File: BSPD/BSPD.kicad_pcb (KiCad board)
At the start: 2 copper layers, 160 x 124.7 mm, 41 parts, among them J1 DT13-48PABCD-R015, K1 Latching Relay, Q1 STS6NF20V, Q2 STS6NF20V, Q3 STS6NF20V, U1 LM7805CT, U10 DK1A1B-12V, U11 NSL-32, U12 LM555N, U13 LM7805CT, U2 OP AMP, U3 OP AMP, U4 Inverter (Not Gate), U5 2x4 OR GATE, U6 LM555N, U7 NSL-32, U8 NAND, U9 AND GATE

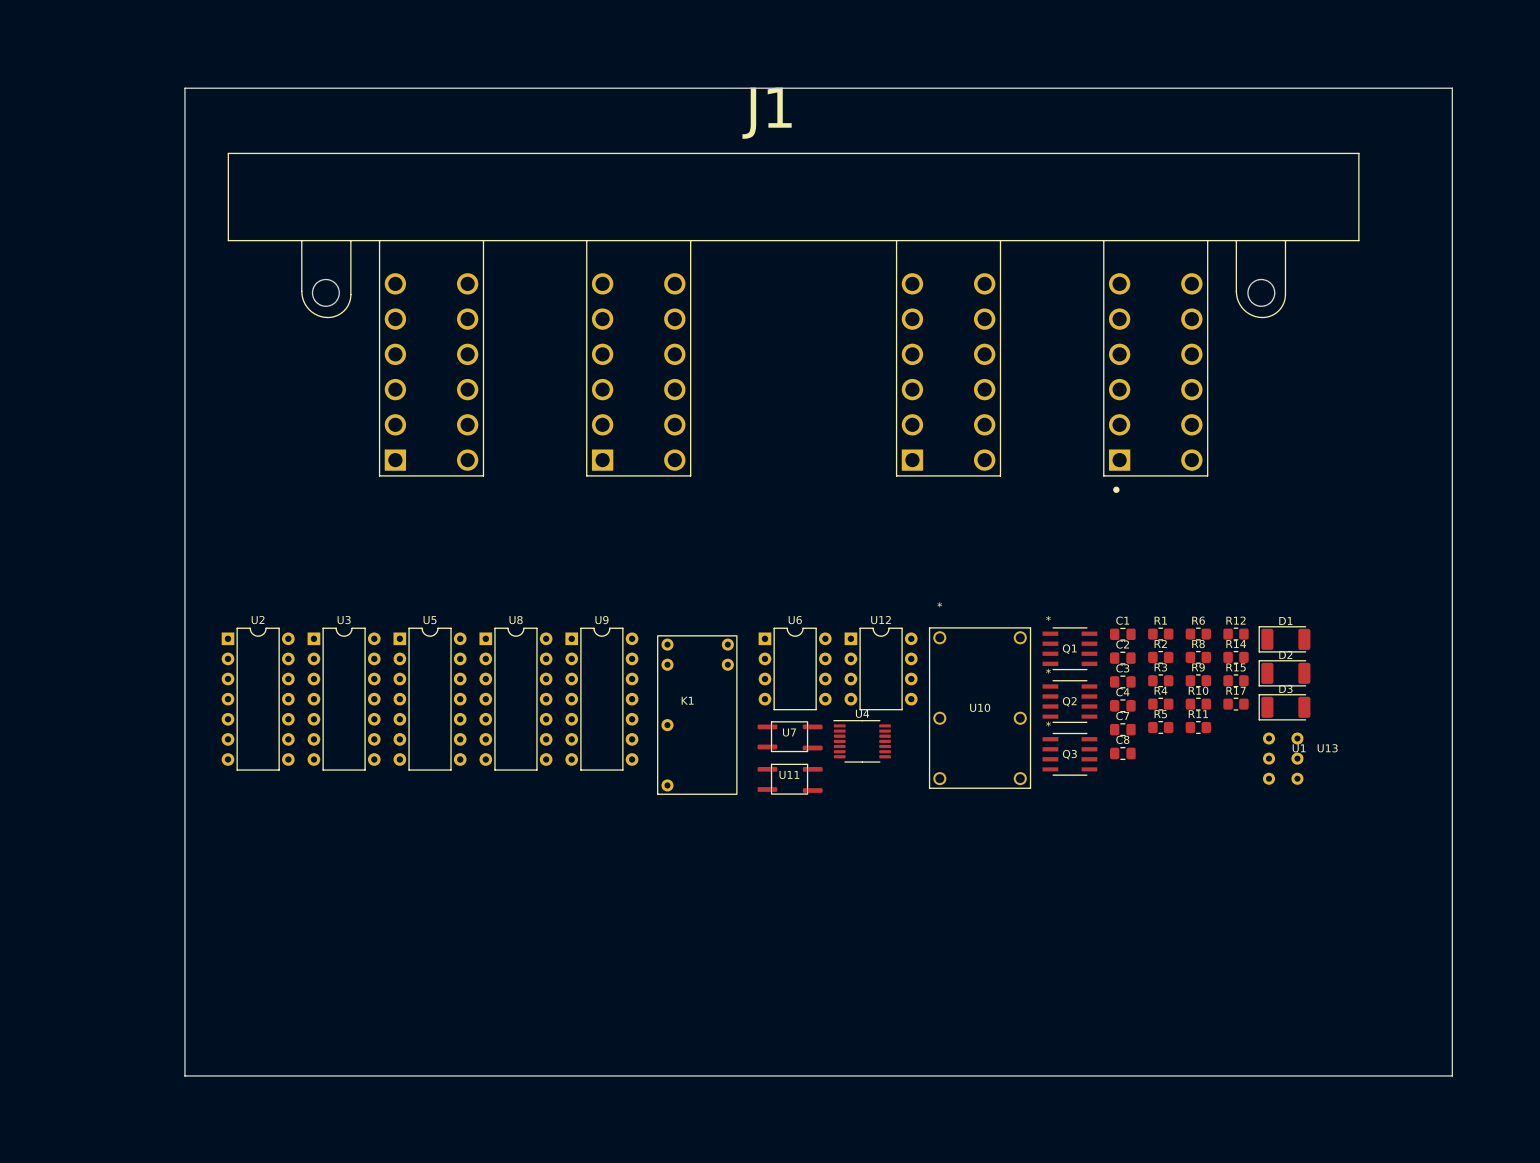
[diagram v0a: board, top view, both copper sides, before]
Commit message: 1/2 BSPD Circuitry
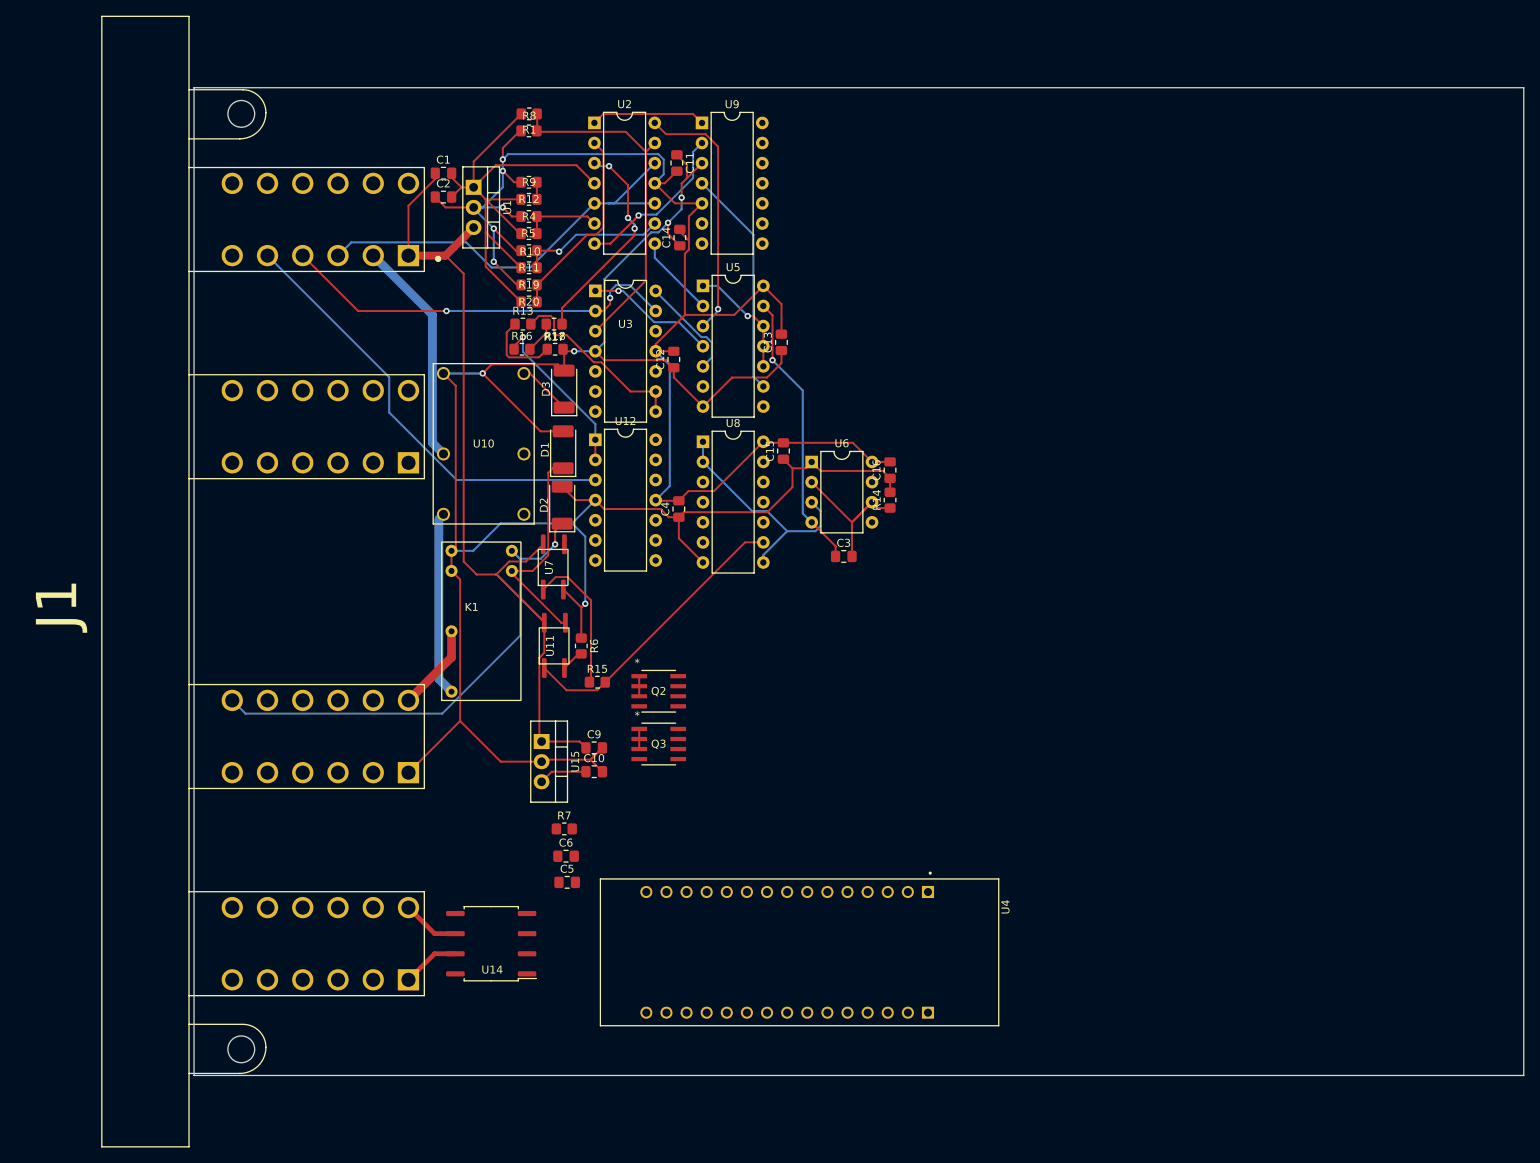
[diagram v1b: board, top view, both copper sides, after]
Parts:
- removed C7: 330nf, Capacitor_SMD:C_0805_2012Metric_Pad1.18x1.45mm_HandSolder
- removed C8: 100nf, Capacitor_SMD:C_0805_2012Metric_Pad1.18x1.45mm_HandSolder
- removed Q1: STS6NF20V, 1FS_2_Global_Footprint_Library:SO-8_STM
- removed R2: 18k, Resistor_SMD:R_0805_2012Metric_Pad1.20x1.40mm_HandSolder
- removed R3: 2.7k, Resistor_SMD:R_0805_2012Metric_Pad1.20x1.40mm_HandSolder
- removed U13: LM7805CT, 1FS_2_Global_Footprint_Library:Basic 3 Hole
- added C10: 0.33µF, Capacitor_SMD:C_0805_2012Metric_Pad1.18x1.45mm_HandSolder, F.Cu at (77.6, 109.2)
- added C11: 100nf, Capacitor_SMD:C_0805_2012Metric_Pad1.18x1.45mm_HandSolder, F.Cu at (88.0, 32.4)
- added C12: 100nf, Capacitor_SMD:C_0805_2012Metric_Pad1.18x1.45mm_HandSolder, F.Cu at (87.6, 57.2)
- added C13: 100nf, Capacitor_SMD:C_0805_2012Metric_Pad1.18x1.45mm_HandSolder, F.Cu at (101.2, 55.0)
- added C14: 100nf, Capacitor_SMD:C_0805_2012Metric_Pad1.18x1.45mm_HandSolder, F.Cu at (88.4, 41.8)
- added C15: 100nf, Capacitor_SMD:C_0805_2012Metric_Pad1.18x1.45mm_HandSolder, F.Cu at (101.5, 68.7)
- added C16: 100nf, Capacitor_SMD:C_0805_2012Metric_Pad1.18x1.45mm_HandSolder, F.Cu at (114.9, 71.1)
- added C5: 100nF, Capacitor_SMD:C_0805_2012Metric_Pad1.18x1.45mm_HandSolder, F.Cu at (74.2, 123.2)
- added C6: 100nF, Capacitor_SMD:C_0805_2012Metric_Pad1.18x1.45mm_HandSolder, F.Cu at (74.0, 119.9)
- added C9: 0.33µF, Capacitor_SMD:C_0805_2012Metric_Pad1.18x1.45mm_HandSolder, F.Cu at (77.6, 106.2)
- added R13: 39k, Resistor_SMD:R_0805_2012Metric_Pad1.20x1.40mm_HandSolder, F.Cu at (68.6, 52.7)
- added R16: 39k, Resistor_SMD:R_0805_2012Metric_Pad1.20x1.40mm_HandSolder, F.Cu at (68.5, 55.9)
- added R18: 1M, Resistor_SMD:R_0805_2012Metric_Pad1.20x1.40mm_HandSolder, F.Cu at (72.6, 55.9)
- added R19: 22k 1%, Resistor_SMD:R_0805_2012Metric_Pad1.20x1.40mm_HandSolder, F.Cu at (69.4, 47.8)
- added R20: 18k 1%, Resistor_SMD:R_0805_2012Metric_Pad1.20x1.40mm_HandSolder, F.Cu at (69.4, 49.9)
- added R7: 120, Resistor_SMD:R_0805_2012Metric_Pad1.20x1.40mm_HandSolder, F.Cu at (73.8, 116.4)
- added U14: ISO1050DUB, Package_SO:SOP-8_6.62x9.15mm_P2.54mm, F.Cu at (64.6, 130.9)
- added U15: LM7809_TO220, Package_TO_SOT_THT:TO-220-3_Vertical, F.Cu at (70.9, 105.4)
- C4: value 1uf -> 100nf
- R17: value 2.4M -> 1M
- U1: footprint 1FS_2_Global_Footprint_Library:Basic 3 Hole -> Package_TO_SOT_THT:TO-220-3_Vertical
- U12: value LM555N -> OP AMP; footprint Package_DIP:DIP-8_W7.62mm -> Package_DIP:DIP-14_W7.62mm
- U4: value Inverter (Not Gate) -> NUCLEO-L432KC; footprint Package_SO:TSSOP-14_4.4x5mm_P0.65mm -> 1FS_2_Global_Footprint_Library:MODULE_NUCLEO-L432KC
- moved U1 123.6 mm to (62.4, 35.4), turned to -90 degrees
- moved R8 108.8 mm to (69.4, 26.2), turned to 180 degrees
- moved R9 105.4 mm to (69.3, 34.8), turned to 180 degrees
- moved R12 104.8 mm to (69.3, 37.0)
- moved C1 103.7 mm to (58.5, 33.7)
- moved C2 103.7 mm to (58.5, 36.7)
- moved R11 102.5 mm to (69.4, 45.6), turned to 180 degrees
- moved R10 102.1 mm to (69.3, 43.4)
- moved R1 102.0 mm to (69.3, 28.3)
- moved R5 101.3 mm to (69.3, 41.3), turned to 180 degrees
- moved R4 100.8 mm to (69.3, 39.1)
- moved D3 99.6 mm to (73.8, 60.9), turned to 90 degrees
- moved R17 98.6 mm to (72.5, 52.7), turned to 180 degrees
- moved D1 94.3 mm to (73.7, 68.6), turned to 90 degrees
- moved D2 93.8 mm to (73.5, 75.6), turned to 90 degrees
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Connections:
- net /4.1V renamed /Brake Threshhold (4.1V)
- net Net-(U2-Pad14) renamed /BrkSenShort
- net Net-(U2-Pad8) renamed /BrkSenOpen
- net Net-(U3-Pad1) renamed /CurSenShort
- net Net-(U3-Pad14) renamed /CurSenOpen
- C3 pad 1: Net-(U6-R) -> /BSPD Fault
- C4 pad 1: +5V -> GND
- C4 pad 2: Net-(U12-THR) -> +5V
- D1 pad 2: Net-(D1-A) -> GND
- J1 pad A10: /BMS_FAULT 3.3V -> unconnected-(J1-PadA10)
- J1 pad A11: /BMS Light Low Side -> unconnected-(J1-PadA11)
- J1 pad A12: /IMD Light Low Side -> unconnected-(J1-PadA12)
- J1 pad A2: unconnected-(J1-PadA2) -> /Shutdown In
- J1 pad A6: /SH_RESET -> unconnected-(J1-PadA6)
- J1 pad A8: /Shutdown In -> unconnected-(J1-PadA8)
- J1 pad A9: /IMD_FAULT -> unconnected-(J1-PadA9)
- J1 pad B1: unconnected-(J1-PadB1) -> /CAN_Tel_H
- J1 pad B12: unconnected-(J1-PadB12) -> /CAN_Tel_L
- J1 pad D10: unconnected-(J1-PadD10) -> /BMS Light Low Side
- J1 pad D11: unconnected-(J1-PadD11) -> /IMD Light Low Side
- J1 pad D12: unconnected-(J1-PadD12) -> /Shutdown Out
- J1 pad D3: /Shutdown Out -> unconnected-(J1-PadD3)
- J1 pad D7: unconnected-(J1-PadD7) -> /SH_RESET
- J1 pad D8: unconnected-(J1-PadD8) -> /IMD_FAULT 5V
- J1 pad D9: unconnected-(J1-PadD9) -> /BMS_FAULT 5V
- K1 pad 2: Net-(D1-A) -> GND
- R15 pad 2: /BSPD Fault -> /BSPD Fault Post Timer
- R17 pad 1: Net-(U12-THR) -> /Current Sensor Differential
- R17 pad 2: GND -> /Current Vref Op
- U11 pad 1: Net-(U11-A) -> /BSPD Fault Post Timer
- U12 pad 1: GND -> /Current Vref Buffered
- U12 pad 2: Net-(U12-THR) -> /Current Vref Buffered
- U12 pad 3: /IMD Latch Delay -> /Current Vref
- U12 pad 4: +5V -> GND
- U12 pad 6: Net-(U12-THR) -> unconnected-(U12-Pad6)
- U12 pad 8: +5V -> unconnected-(U12-Pad8)
- U2 pad 2: /Current Vref -> /2.25V
- U2 pad 3: /Current Output -> /Current Sensor Differential
- U2 pad 5: /Current Output -> /Brake Output
- U3 pad 10: /BMS_FAULT 3.3V -> /Current Output
- U3 pad 5: unconnected-(U3-Pad5) -> /Current Vref Op
- U3 pad 6: unconnected-(U3-Pad6) -> /Current Output Op
- U3 pad 7: unconnected-(U3-Pad7) -> /Current Sensor Differential
- U3 pad 8: /BMS_FAULT 5V -> /Current Output Buffered
- U3 pad 9: /3V -> /Current Output Buffered
- U5 pad 13: Net-(U6-R) -> /BSPD Fault
- U6 pad 4: Net-(U6-R) -> /BSPD Fault
- U6 pad 8: Net-(U6-R) -> +5V
- U8 pad 1: /BSPD_FAULT -> Net-(U6-Q)
- U8 pad 14: (no net) -> +5V
- U8 pad 2: /IMD_FAULT 5V -> Net-(U6-Q)
- U8 pad 7: (no net) -> GND
- U8 pad 8: /BMS_FAULT 5V -> Net-(U6-Q)
- U8 pad 9: Net-(U11-A) -> /BSPD Fault Post Timer
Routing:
- net GND: track 0.00 -> 355.1 mm, vias 0 -> 5
- net +5V: track 0.00 -> 177.4 mm, vias 0 -> 5
- net +12V: track 0.00 -> 112.0 mm
- net /SH_RESET: track 0.00 -> 61.9 mm, vias 0 -> 1
- net /Current Vref: track 0.00 -> 55.7 mm
- net /Brake Output: track 0.00 -> 53.3 mm
- net /Current Output: track 0.00 -> 51.1 mm, vias 0 -> 2
- net /4.5V: track 0.00 -> 43.9 mm
- net /BSPD Fault Post Timer: track 0.00 -> 36.6 mm
- net /BSPD Fault: track 0.00 -> 35.4 mm, vias 0 -> 1
- net /BrkSenShort: track 0.00 -> 32.7 mm, vias 0 -> 1
- net Net-(U6-Q): track 0.00 -> 29.9 mm
- net Net-(U5-Pad9): track 0.00 -> 28.9 mm
- net /Shutdown In: track 0.00 -> 28.7 mm
- net Net-(D1-K): track 0.00 -> 27.6 mm
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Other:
- board size 160 x 124.7 mm -> 167.9 x 124.7 mm
